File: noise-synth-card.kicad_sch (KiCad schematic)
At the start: 40 parts, among them J1 CVpitch, J2 FM in, M1 imogen-wren-card, Q1 BC558, Q2 BC548, U1 40106, U2 TL074, U3 HEF4093B

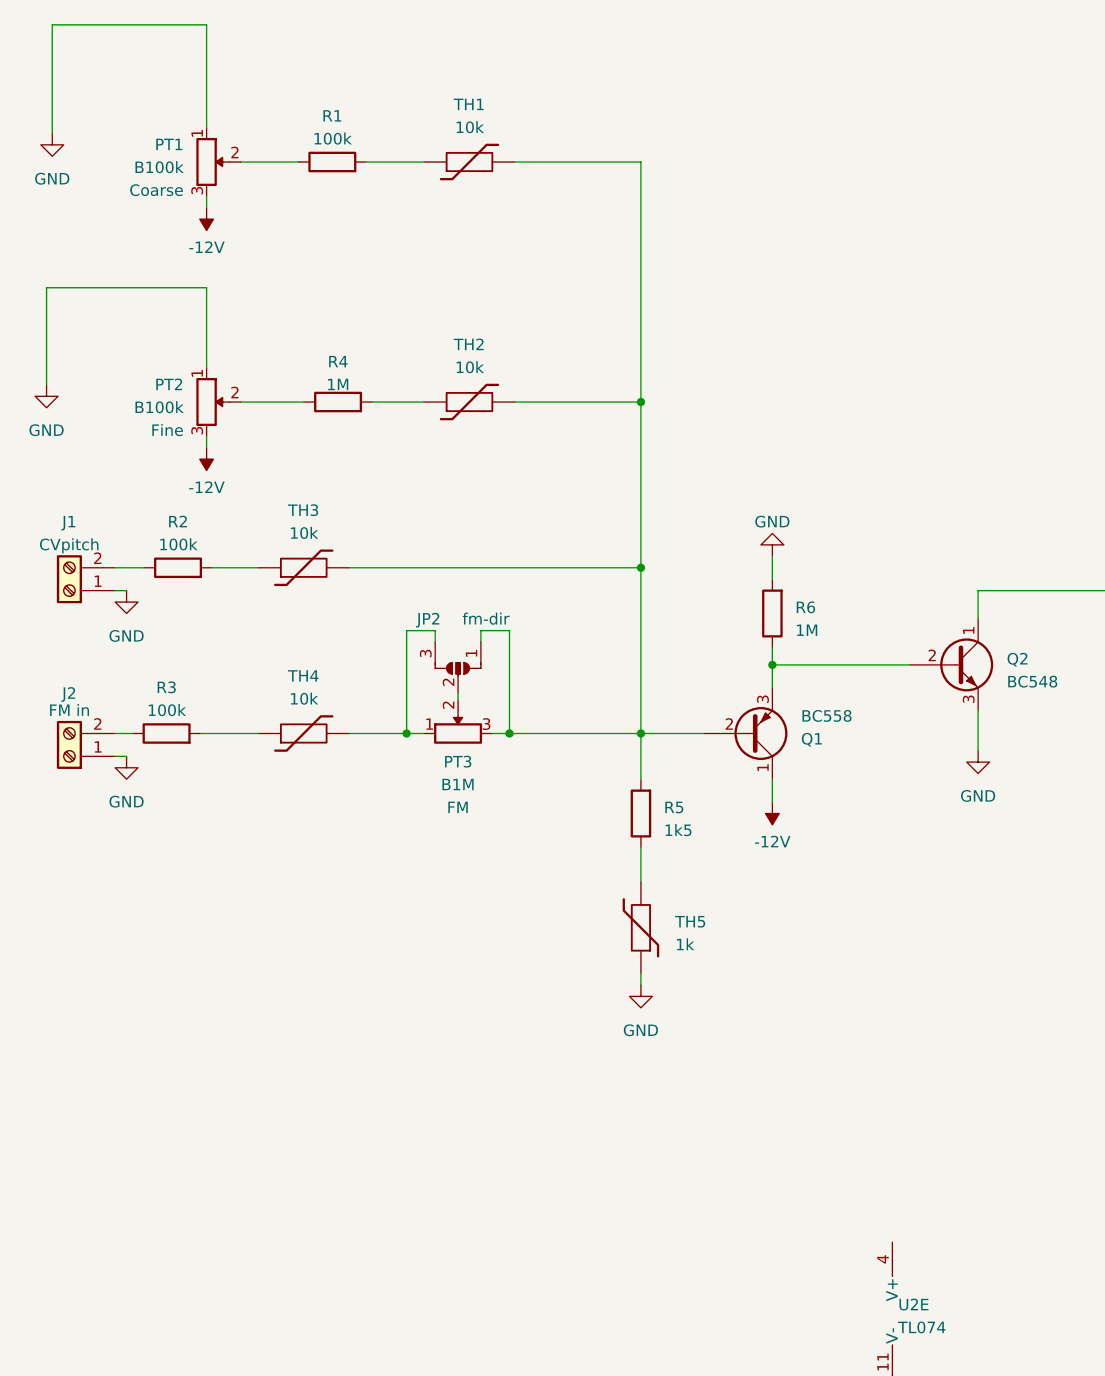
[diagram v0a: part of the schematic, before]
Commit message: dgfhdh
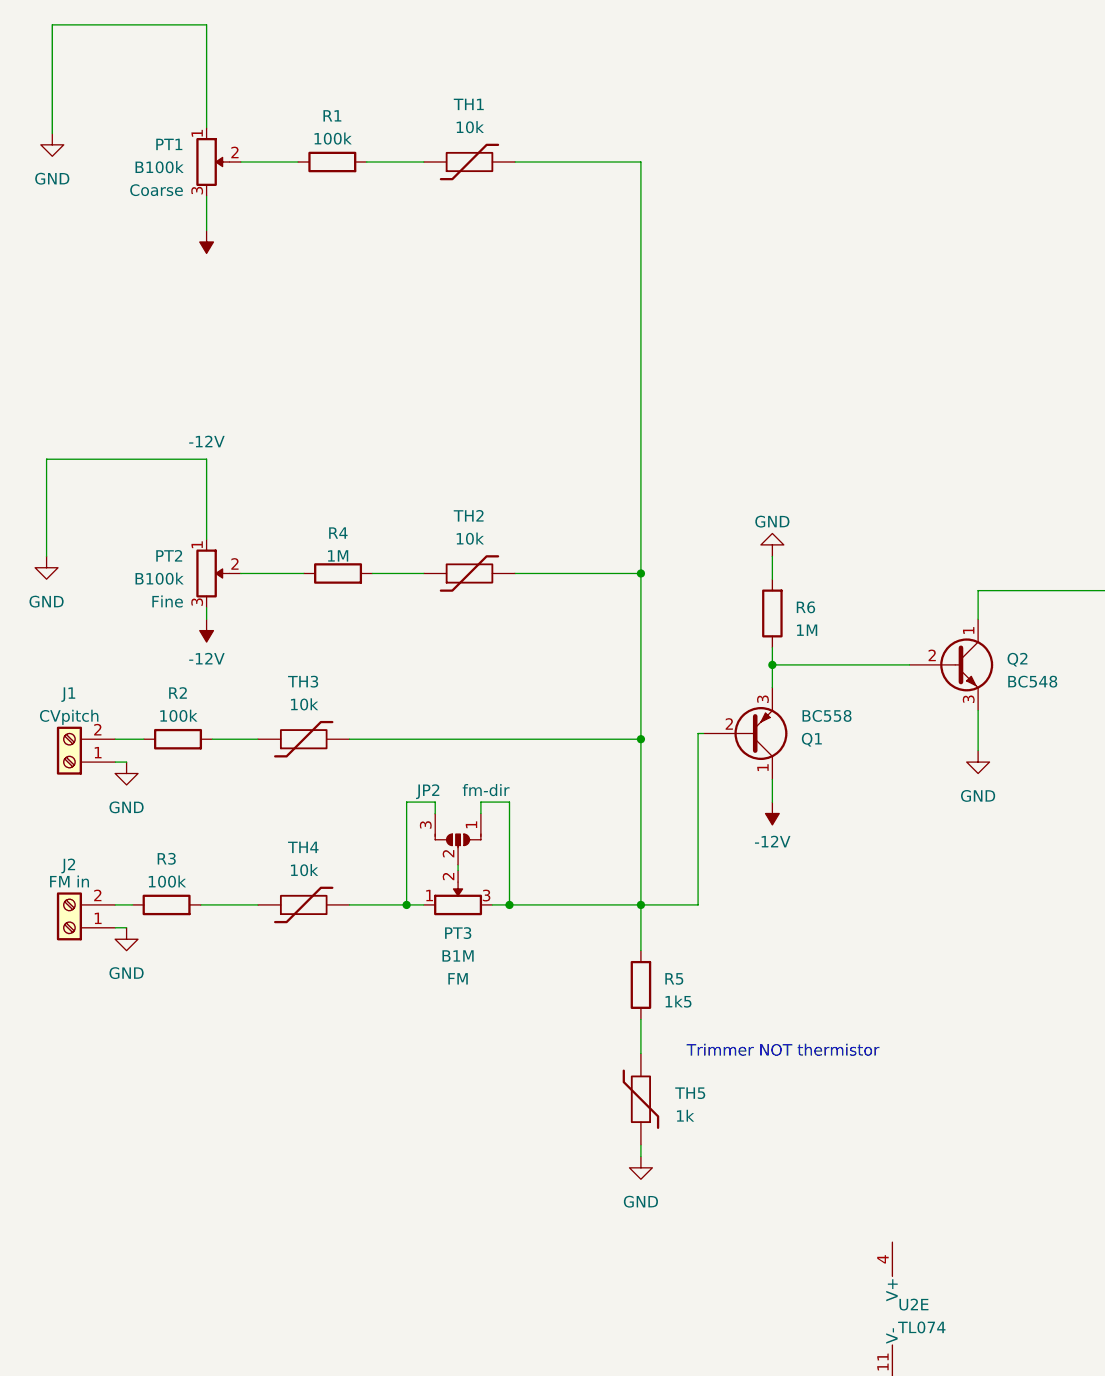
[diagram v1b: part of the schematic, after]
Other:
- note added: "Trimmer NOT thermistor"
- moved on the sheet: J1, J2, JP2, PT2, PT3, R2, R3, R4, R5, TH2, TH3, TH4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
